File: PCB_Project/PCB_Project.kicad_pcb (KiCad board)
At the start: 2 copper layers, 55 x 55 mm, 39 parts, among them J2 ZE27-O3, J3 Motor_Connector, J4 Motor_Connector, J5 Motor_Connector, J6 Motor_Connector, Q1 BSS138, Q2 BSS138, Q3 MMBT2222A, Q4 MMBT2222A

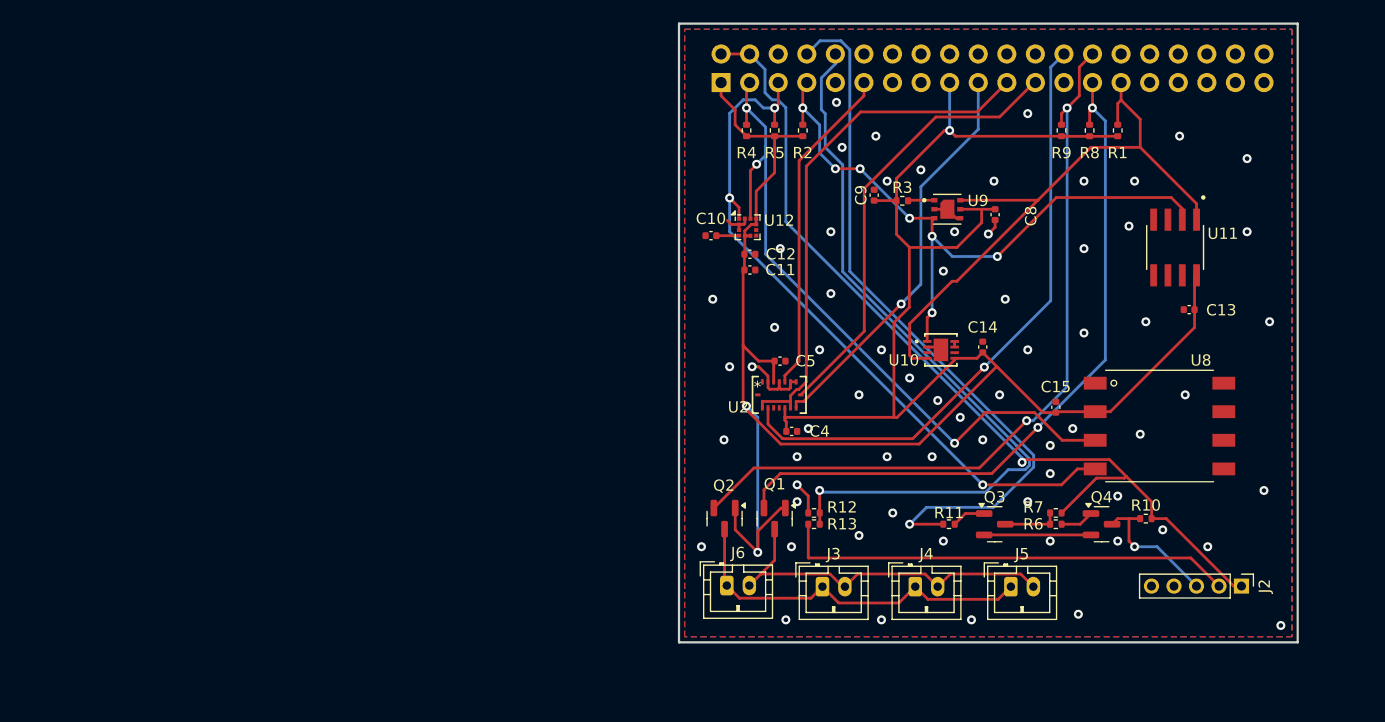
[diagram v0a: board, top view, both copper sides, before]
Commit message: working on final board
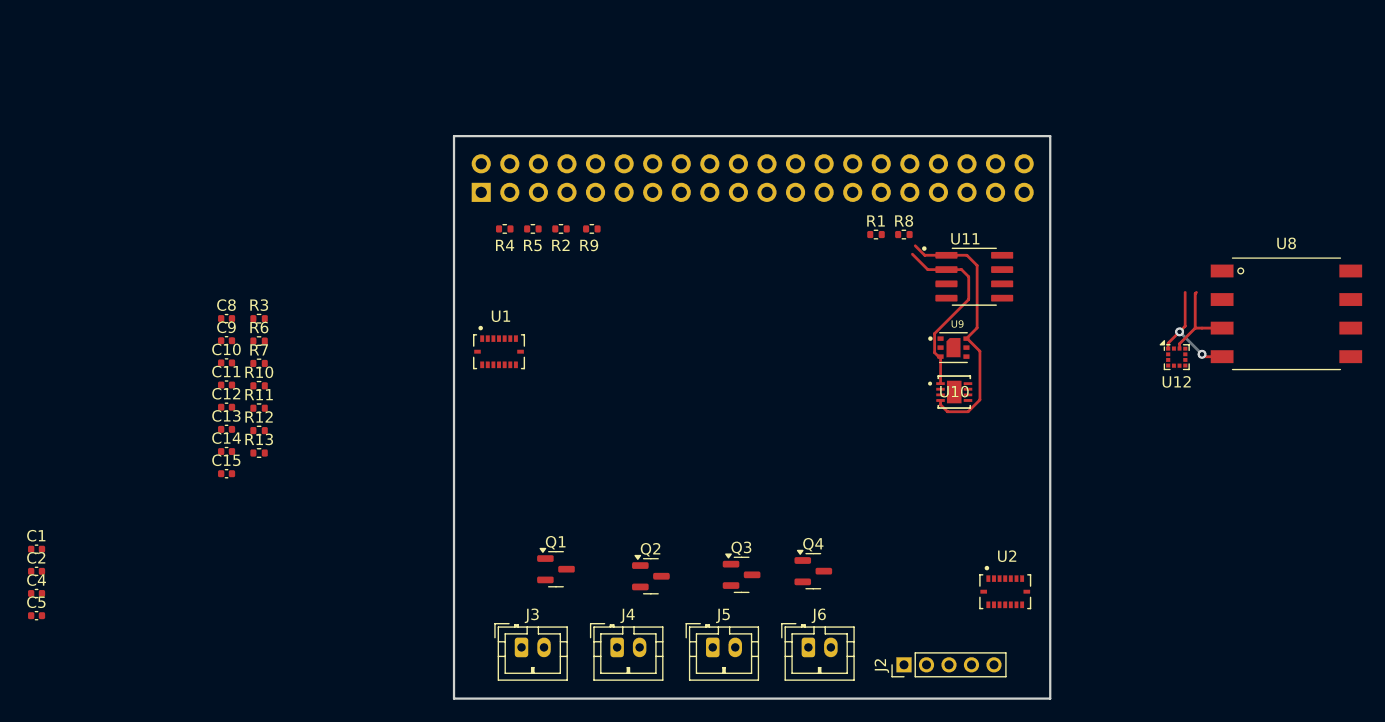
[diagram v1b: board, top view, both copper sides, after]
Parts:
- added C1: 100nF, Capacitor_SMD:C_0402_1005Metric, F.Cu at (56.4, 104.2)
- added C2: 100nF, Capacitor_SMD:C_0402_1005Metric, F.Cu at (56.4, 106.2)
- added U1: ~, Sensor:PQFN50P450X300X100-16N, F.Cu at (97.5, 86.7)
- U11: footprint Sensor:SOIC127P600X175-8N_ADT7410TRZ-REEL -> Sensor:SOIC127P600X175-8N
- U2: footprint Sensor:QFN_BMI085_BOS -> Sensor:PQFN50P450X300X100-16N
- moved C13 86.2 mm to (73.3, 93.6), turned to 0 degrees
- moved R10 79.7 mm to (76.2, 89.7)
- moved C15 74.0 mm to (73.3, 97.5), turned to 0 degrees
- moved R6 72.7 mm to (76.2, 85.7)
- moved R7 72.1 mm to (76.2, 87.7)
- moved C5 69.9 mm to (56.4, 110.1)
- moved C8 68.9 mm to (73.3, 83.7), turned to 0 degrees
- moved C4 68.7 mm to (56.4, 108.2)
- moved C14 67.9 mm to (73.3, 95.5), turned to 0 degrees
- moved R11 62.2 mm to (76.2, 91.7), turned to 0 degrees
- moved C9 59.0 mm to (73.3, 85.7), turned to 0 degrees
- moved R3 58.1 mm to (76.2, 83.7)
- moved R12 49.9 mm to (76.2, 93.7)
- moved R13 49.7 mm to (76.2, 95.7), turned to 0 degrees
- moved C12 48.5 mm to (73.3, 91.6)
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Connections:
- net SDI_1 renamed MOSI_1
- net SDO_1 renamed MISO_1
- U4 pad 10: Pi_RX -> I2C_SCL_M
- U4 pad 12: nCS_2 -> unconnected-(U4-GPIO_18-Pad12)
- U4 pad 26: CSB_Accel_BMI088 -> unconnected-(U4-GPIO_7-Pad26)
- U4 pad 27: I2C_SDA_M -> Pi_TX
- U4 pad 28: I2C_SCL_M -> Pi_RX
- U4 pad 31: unconnected-(U4-GPIO_6-Pad31) -> I2C_SDA_M
- U4 pad 35: SDO_2 -> MISO_2
- U4 pad 36: unconnected-(U4-GPIO_16-Pad36) -> CSB_Accel_BMI088
- U4 pad 38: SDI_2 -> MOSI_2
- U4 pad 40: SCLK_2 -> SCK_2
- U4 pad 8: Pi_TX -> unconnected-(U4-GPIO_14-Pad8)
- U4 pad 9: GND -> unconnected-(U4-GND-Pad9)
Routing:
- net +3V3: track 204.8 -> 0.00 mm, vias 3 -> 0
- net +5V: track 81.4 -> 0.00 mm, vias 1 -> 0
- net I2C_SCL_M: track 68.1 -> 0.00 mm, vias 2 -> 0
- net Pi_RX: track 67.5 -> 0.00 mm, vias 1 -> 0
- net Pi_TX: track 64.6 -> 0.00 mm, vias 1 -> 0
- net I2C_SDA_M: track 63.5 -> 0.00 mm, vias 2 -> 0
- net I2C_SDA_1: track 63.0 -> 8.01 mm, vias 3 -> 0
- net CSB_Accel_BMI088: track 54.6 -> 0.00 mm, vias 1 -> 0
- net I2C_SCL_1: track 63.8 -> 10.3 mm, vias 3 -> 2
- net MISO_1: track 46.1 -> 0.00 mm
- net I2C_SDA_2: track 58.9 -> 17.1 mm, vias 7 -> 0
- net Pi_RX_5V: track 40.5 -> 0.00 mm
- net SCK_1: track 39.8 -> 0.00 mm
- net MOSI_1: track 36.0 -> 0.00 mm, vias 1 -> 0
- net I2C_SCL_M_5V: track 33.4 -> 0.00 mm
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- removed copper zone on B.Cu, net GND
- removed copper zone on F.Cu, net GND
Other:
- board size 55 x 55 mm -> 53 x 50 mm
